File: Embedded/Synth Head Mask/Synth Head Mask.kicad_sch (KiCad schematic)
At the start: 13 parts, among them J1 JST [S], J2 JST [M], J3 JST [F], J4 JST [F], J5 JST [B], J6 JST [K], Q1 BSS138, Q2 AS2302, U1 FFC [M], U2 FFC [S]

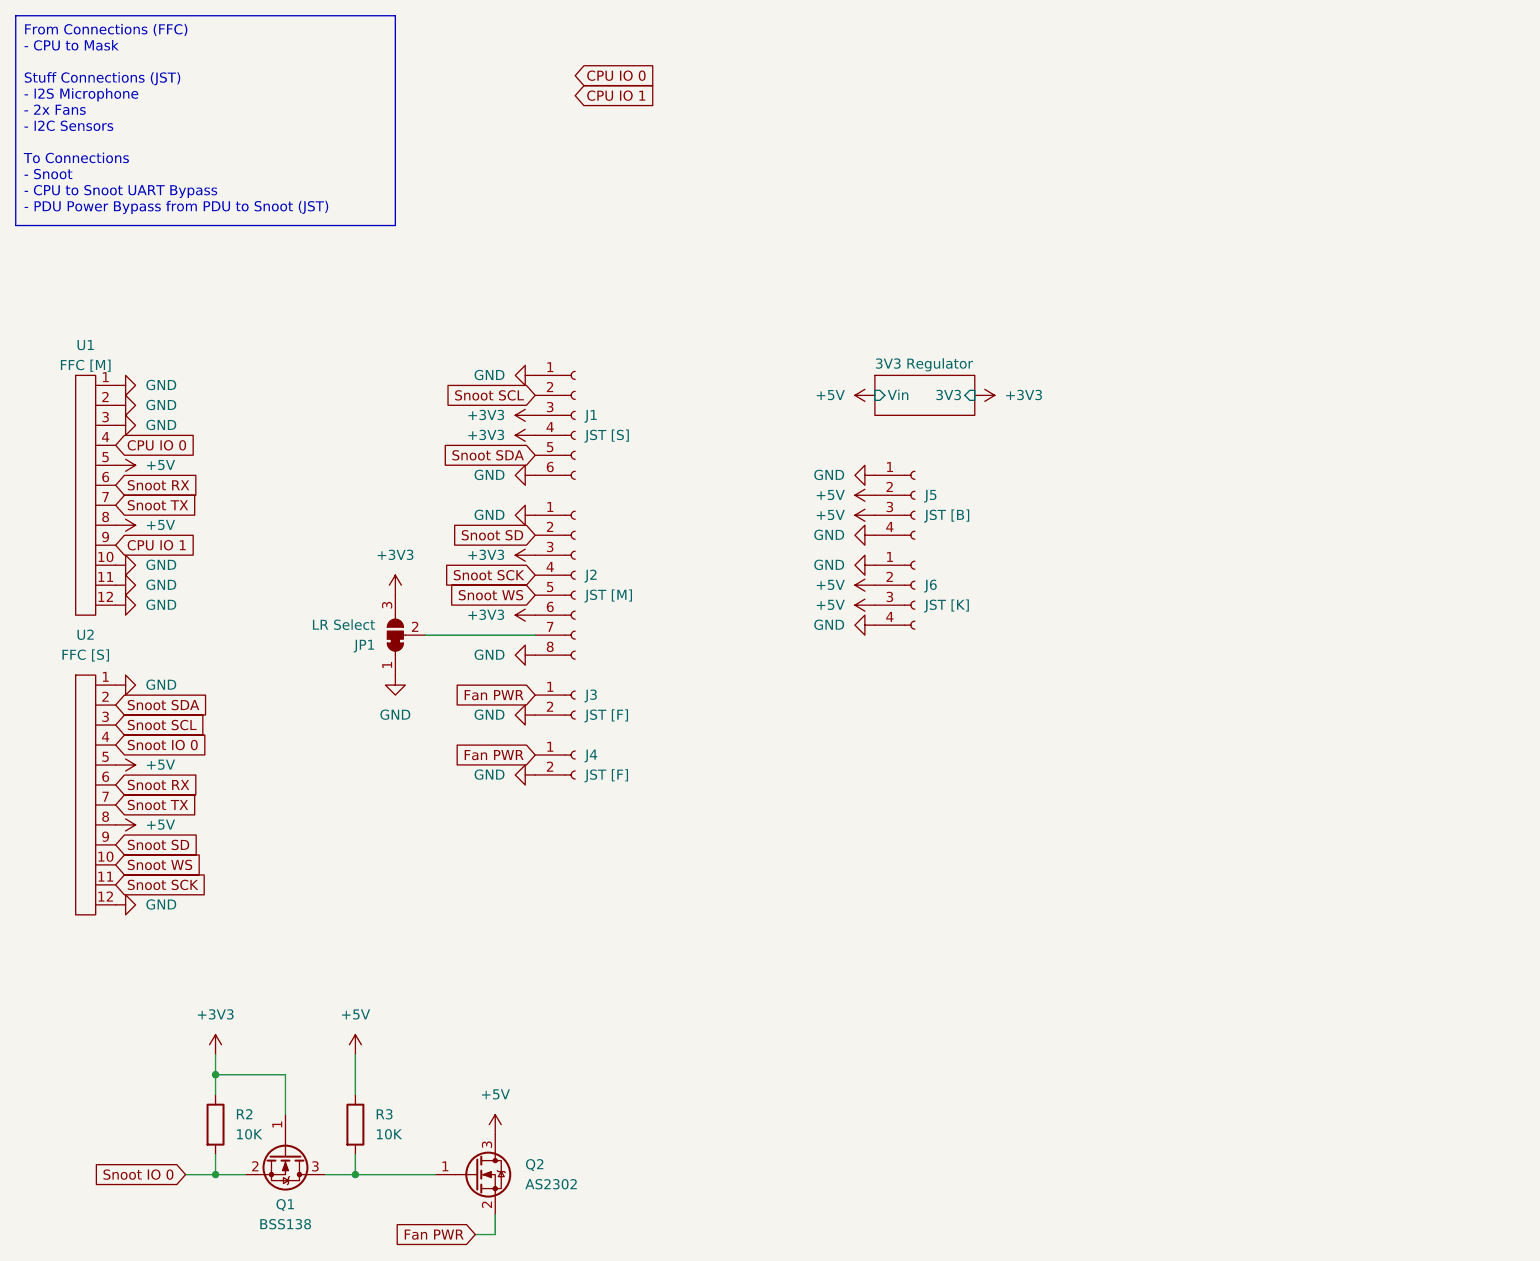
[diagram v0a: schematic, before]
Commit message: Prepared All Main Boards for PCB Creation
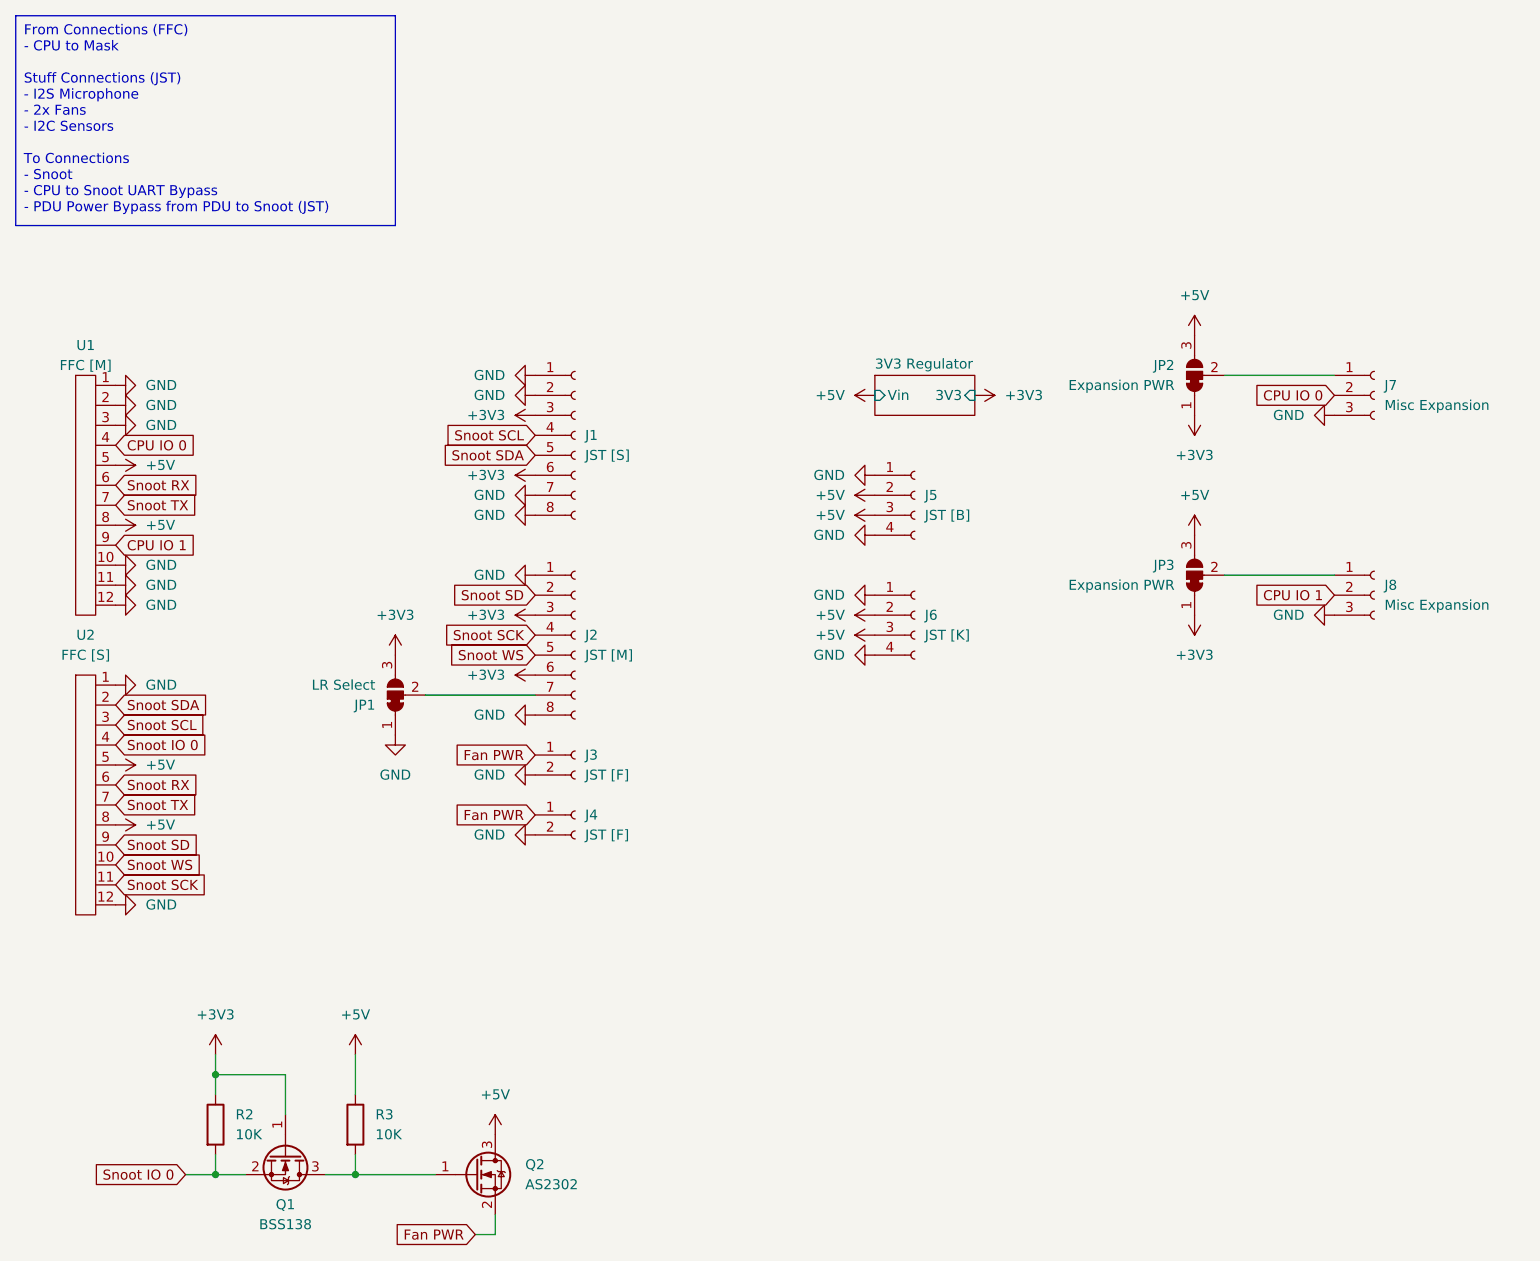
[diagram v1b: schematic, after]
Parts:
- removed J1: JST [S], symbol Connector:Conn_01x06_Socket
- added J1: JST [S], Connector_Molex:Molex_PicoBlade_53047-0810_1x08_P1.25mm_Vertical, symbol Connector:Conn_01x08_Socket
- added J7, J8: Misc Expansion, Connector_PinHeader_2.54mm:PinHeader_1x03_P2.54mm_Vertical, symbol Connector:Conn_01x03_Socket
- added JP2, JP3: Expansion PWR, Jumper:SolderJumper-3_P1.3mm_Bridged2Bar12_Pad1.0x1.5mm, symbol Jumper:SolderJumper_3_Bridged12
- J2: footprint (none) -> Connector_Molex:Molex_PicoBlade_53047-0810_1x08_P1.25mm_Vertical
- J3, J4: footprint (none) -> Connector_Molex:Molex_PicoBlade_53047-0210_1x02_P1.25mm_Vertical
- J5, J6: footprint (none) -> Connector_Molex:Molex_PicoBlade_53047-0410_1x04_P1.25mm_Vertical
- JP1: footprint (none) -> Jumper:SolderJumper-3_P1.3mm_Bridged12_RoundedPad1.0x1.5mm
- R2, R3: footprint (none) -> Resistor_SMD:R_0603_1608Metric_Pad0.98x0.95mm_HandSolder
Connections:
- net +3V3: now also J1.3 (Pin_3), J1.6 (Pin_6), JP2.1 (A), JP3.1 (A)
- net +5V: now also JP2.3 (B), JP3.3 (B)
- net CPU IO 0: now also J7.2 (Pin_2)
- net CPU IO 1: now also J8.2 (Pin_2)
- net GND: now also J1.1 (Pin_1), J1.2 (Pin_2), J1.7 (Pin_7), J1.8 (Pin_8), J7.3 (Pin_3), J8.3 (Pin_3)
- net Snoot SCL: now also J1.4 (Pin_4)
- net Snoot SDA: now also J1.5 (Pin_5)
- new net: J8.1 (Pin_1), JP3.2 (C)
- new net: J7.1 (Pin_1), JP2.2 (C)
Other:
- moved on the sheet: J2, J3, J4, J6, JP1
